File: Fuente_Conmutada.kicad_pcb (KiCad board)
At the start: 2 copper layers, 97.3 x 97.3 mm, 48 parts, among them J1 Terminal_220v, J2 Terminal_12v, J3 Vout, Q1 IRF840, Q2 IRF840, T1 Transformer_1P_SS, U1 TL494, U2 IR2110

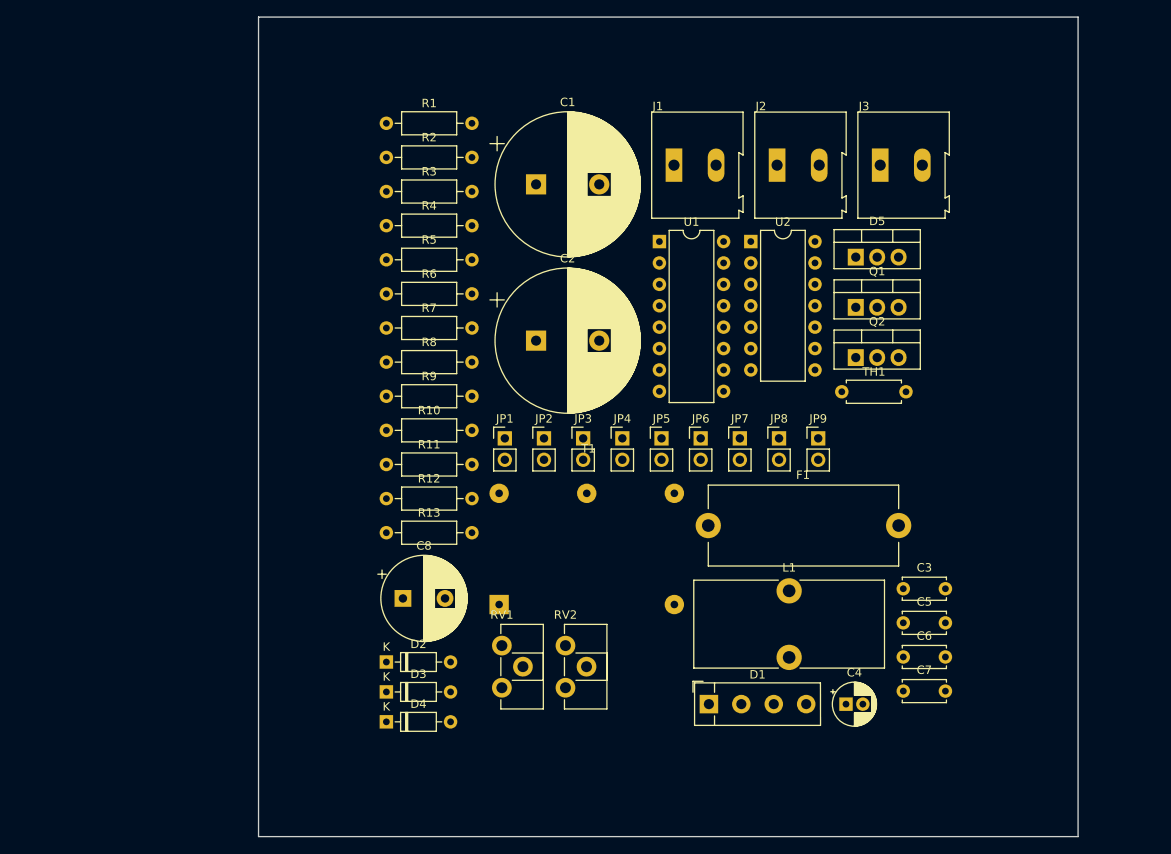
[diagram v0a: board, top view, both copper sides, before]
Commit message: dawd
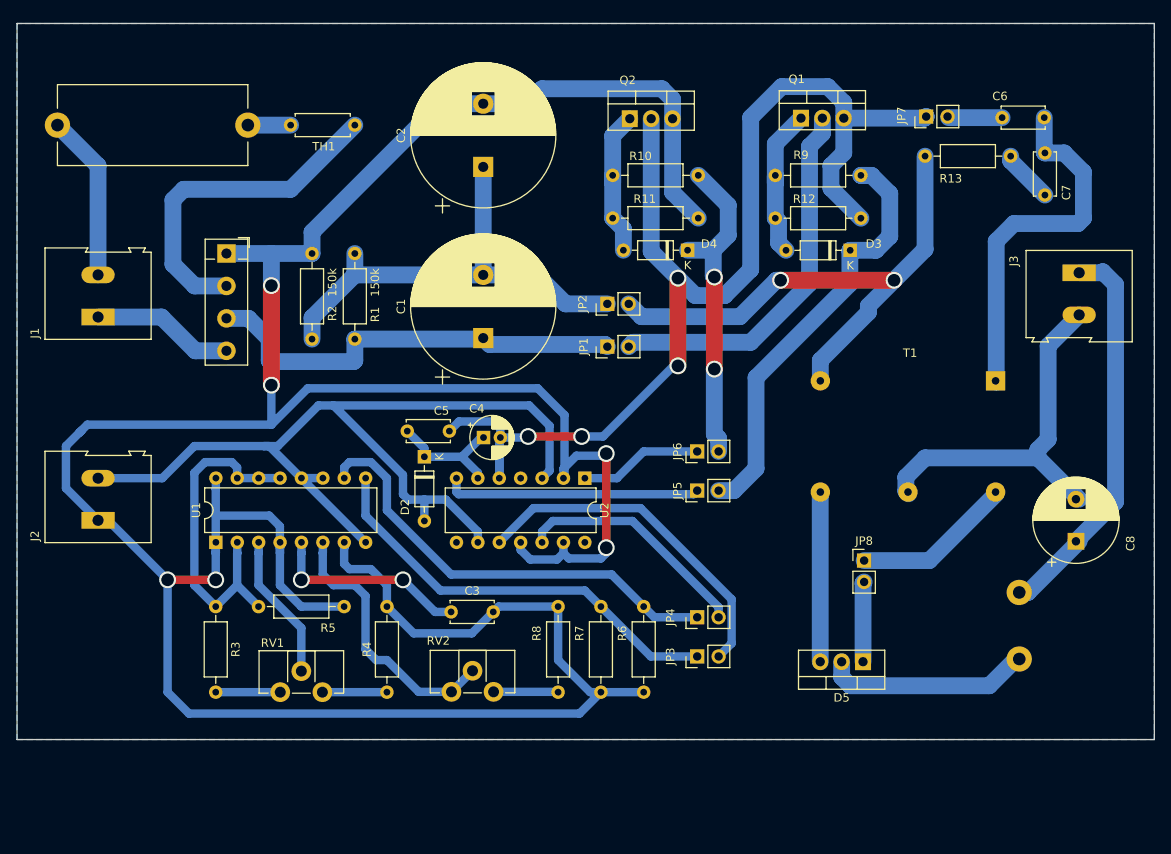
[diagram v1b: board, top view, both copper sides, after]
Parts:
- removed JP9: Jumper, Connector_PinHeader_2.54mm:PinHeader_1x02_P2.54mm_Vertical
- L1: moved to B.Cu
- moved J2 91.0 mm to (86.6, 109.8), turned to 90 degrees
- moved R13 86.5 mm to (194.9, 66.5), turned to 180 degrees
- moved C8 80.2 mm to (202.7, 112.3), turned to 90 degrees
- moved D1 78.4 mm to (101.9, 78.1), turned to -90 degrees
- moved D3 76.0 mm to (175.9, 77.7), turned to 180 degrees
- moved F1 72.4 mm to (104.4, 62.9), turned to 180 degrees
- moved J1 70.7 mm to (86.6, 85.6), turned to 90 degrees
- moved D4 66.4 mm to (156.6, 77.7), turned to 180 degrees
- moved C6 66.2 mm to (198.9, 62.0), turned to 180 degrees
- moved C7 66.1 mm to (199.0, 66.2), turned to -90 degrees
- moved TH1 65.9 mm to (117.1, 62.9), turned to 180 degrees
- moved R12 65.4 mm to (177.2, 73.9), turned to 180 degrees
- moved U1 63.6 mm to (100.6, 112.4), turned to 90 degrees
- moved C5 63.1 mm to (123.3, 99.2)
- moved R9 62.1 mm to (177.2, 68.8), turned to 180 degrees
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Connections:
- net 1 renamed GND
- net Net-(J1-Pin_2) renamed VAC
- C4 pad 2: Net-(U2-VS) -> Vs
- C5 pad 2: Net-(U2-VS) -> Vs
- D3 pad 1: Net-(D3-K) -> HO
- D4 pad 1: Net-(D4-K) -> LO
- JP2 pad 2: Net-(JP2-B) -> /Punto_medio
- JP3 pad 2: unconnected-(JP3-B-Pad2) -> PWM1
- JP4 pad 2: unconnected-(JP4-B-Pad2) -> PWM2
- JP5 pad 2: unconnected-(JP5-B-Pad2) -> HO
- JP6 pad 2: unconnected-(JP6-B-Pad2) -> LO
- JP7 pad 1: Net-(JP2-B) -> Vs
- Q1 pad 3: Net-(JP2-B) -> Vs
- Q2 pad 2: Net-(JP2-B) -> Vs
- R10 pad 1: Net-(D4-K) -> LO
- R12 pad 1: Net-(D3-A) -> Vs
- R12 pad 2: Net-(JP2-B) -> Net-(D3-A)
- R13 pad 2: Net-(JP2-B) -> /Punto_medio
- R3 pad 1: Net-(U1-1IN-) -> Vref
- R5 pad 1: Net-(U1-1IN-) -> Vref
- R9 pad 1: Net-(D3-K) -> HO
- T1 pad 2: Net-(JP2-B) -> /Punto_medio
- T1 pad 3: Net-(JP9-A) -> Net-(D5-A2)
- U1 pad 13: unconnected-(U1-OUTCTRL-Pad13) -> Vref
- U1 pad 14: unconnected-(U1-REF-Pad14) -> Vref
- U1 pad 15: Net-(U1-1IN-) -> Vref
- U1 pad 2: Net-(U1-1IN-) -> Vref
- U2 pad 10: unconnected-(U2-HIN-Pad10) -> PWM1
- U2 pad 12: unconnected-(U2-LIN-Pad12) -> PWM2
- U2 pad 5: Net-(U2-VS) -> Vs
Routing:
- net GND: track 0.00 -> 388.6 mm, vias 0 -> 6
- net Vs: track 0.00 -> 140.7 mm, vias 0 -> 4
- net +12V: track 0.00 -> 112.6 mm
- net /Punto_medio: track 0.00 -> 65.7 mm, vias 0 -> 2
- net Net-(JP2-A): track 0.00 -> 56.5 mm
- net Net-(JP4-A): track 0.00 -> 53.3 mm
- net Net-(D1-+): track 0.00 -> 51.9 mm
- net HO: track 0.00 -> 51.9 mm
- net Net-(JP3-A): track 0.00 -> 50.8 mm
- net Net-(J3-Pin_1): track 0.00 -> 47.1 mm
- net Net-(JP1-B): track 0.00 -> 44.8 mm
- net 2: track 0.00 -> 44.7 mm
- net Net-(T1-AA): track 0.00 -> 43.5 mm
- net Vref: track 0.00 -> 41.4 mm
- net PWM1: track 0.00 -> 41.2 mm
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- added copper zone on B.Cu, net GND
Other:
- board size 97.3 x 97.3 mm -> 135 x 85 mm
- board text added: "150k"
- board text added: "R1"
- board text added: "R2"
